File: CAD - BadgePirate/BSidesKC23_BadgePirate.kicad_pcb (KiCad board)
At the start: 2 copper layers, 54.8 x 147.9 mm, 75 parts, among them J1 UART, J2 JTAG, J3 Reset Jumper, J4 5v GND, J5 Boot Jumper, J6 USB, SW1 Boot, SW3 SW_Left, SW4 SW_Right, SW5 SW_Center, SW6 SW_Up, SW7 SW_Down, U1 CH340N, U2 ESP32-S3-WROOM-1, U3 TLV1117, U4 LTC4054, X1 sao_v169bis

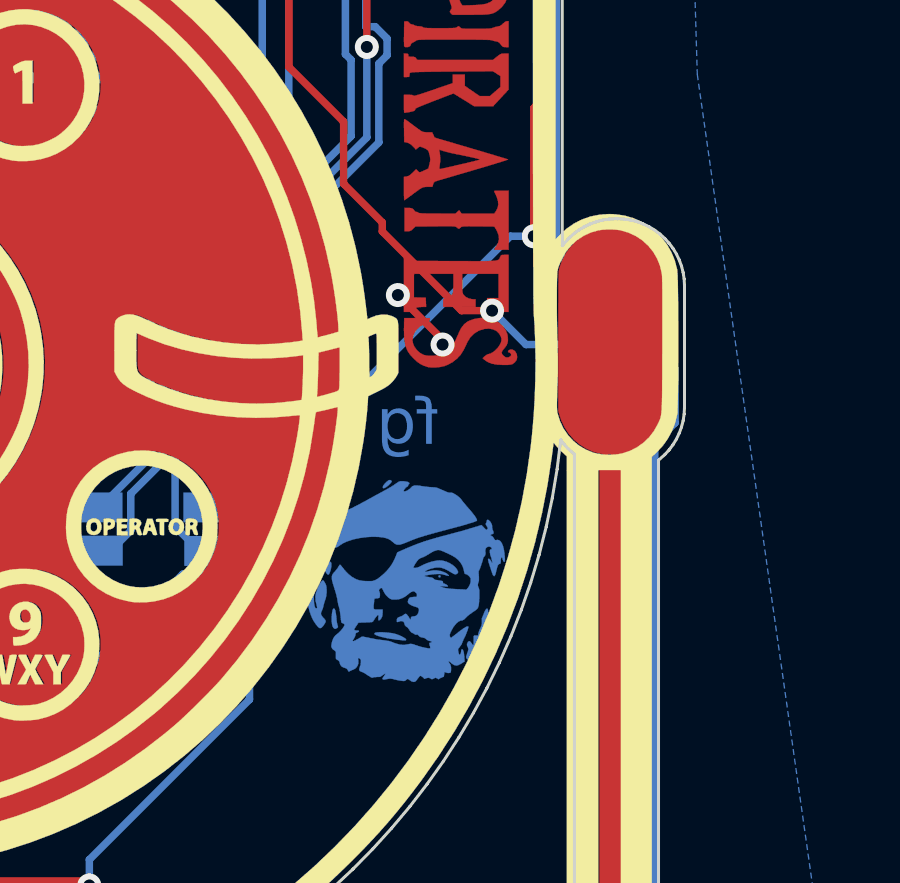
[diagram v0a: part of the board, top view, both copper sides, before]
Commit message: gerberss
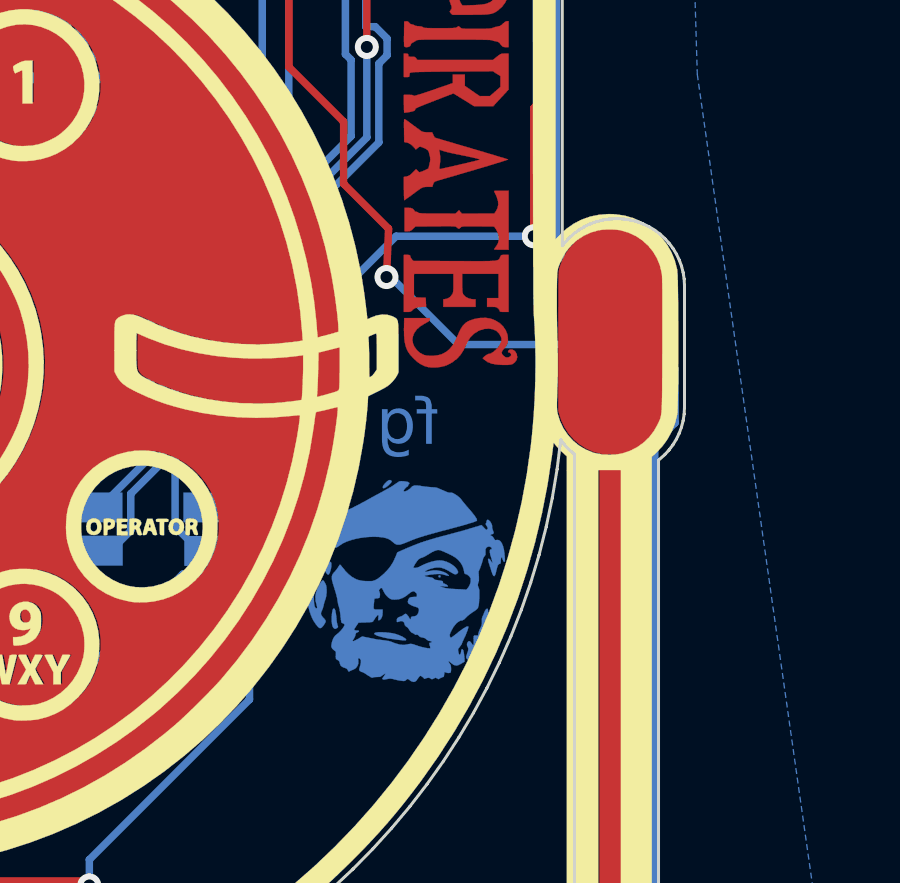
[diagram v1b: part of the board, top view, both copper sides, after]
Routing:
- net GND: track 63.5 -> 61.2 mm, vias 15 -> 13
- net IO02: track 133.7 -> 135.9 mm
- net Boot: track 152.1 -> 152.9 mm
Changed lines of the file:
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@@
   (segment (start 107.14 136.9) (end 108.1 135.94) (width 0.25) (layer "F.Cu") (net 2))
   (segment (start 112.95899 88.630416) (end 111.549074 87.2205) (width 0.25) (layer "F.Cu") (net 2))
-  (segment (start 119.43 109.5) (end 119.43 109.34) (width 0.25) (layer "F.Cu") (net 2))
   (segment (start 89.678075 172.588217) (end 89.35 172.260142) (width 0.25) (layer "F.Cu") (net 2))
   (segment (start 106.2 136.9) (end 107.14 136.9) (width 0.25) (layer "F.Cu") (net 2))
   (segment (start 81.61 79.44) (end 81.18 79.01) (width 0.25) (layer "F.Cu") (net 2))
-  (segment (start 119.43 109.34) (end 117.94 107.85) (width 0.25) (layer "F.Cu") (net 2))
   (segment (start 89.35 171.1) (end 89.82 170.63) (width 0.25) (layer "F.Cu") (net 2))
   (segment (start 100.49 49.59) (end 100.53 49.55) (width 0.25) (layer "F.Cu") (net 2))
@@
   (segment (start 89.35 172.260142) (end 89.35 171.1) (width 0.25) (layer "F.Cu") (net 2))
   (segment (start 92.268217 172.588217) (end 89.678075 172.588217) (width 0.25) (layer "F.Cu") (net 2))
-  (via (at 117.94 107.85) (size 0.8) (drill 0.4) (layers "F.Cu" "B.Cu") (free) (net 2))
   (via (at 89.82 170.63) (size 0.8) (drill 0.4) (layers "F.Cu" "B.Cu") (free) (net 2))
   (via (at 78.92 79.01) (size 0.8) (drill 0.4) (layers "F.Cu" "B.Cu") (free) (net 2))
@@
   (via (at 100.53 49.55) (size 0.8) (drill 0.4) (layers "F.Cu" "B.Cu") (free) (net 2))
   (via (at 88.63 84.41) (size 0.8) (drill 0.4) (layers "F.Cu" "B.Cu") (free) (net 2))
-  (via (at 119.43 109.5) (size 0.8) (drill 0.4) (layers "F.Cu" "B.Cu") (free) (net 2))
   (via (at 106.2 136.9) (size 0.8) (drill 0.4) (layers "F.Cu" "B.Cu") (free) (net 2))
   (via (at 111.549074 87.2205) (size 0.8) (drill 0.4) (layers "F.Cu" "B.Cu") (free) (net 2))
@@
   (segment (start 82.73 115.871517) (end 82.73 119.328041) (width 0.25) (layer "B.Cu") (net 30))
   (segment (start 82.0695 111.49) (end 81.795 111.2155) (width 0.25) (layer "B.Cu") (net 30))
+  (segment (start 102.26972 92.53) (end 102.139719 92.4) (width 0.25) (layer "F.Cu") (net 31))
+  (segment (start 117.56 107.25) (end 117.63 105.64) (width 0.25) (layer "F.Cu") (net 31))
+  (segment (start 101.3 92.4) (end 101.0255 92.6745) (width 0.25) (layer "F.Cu") (net 31))
+  (segment (start 114.31 100.25) (end 114.31 97.939595) (width 0.25) (layer "F.Cu") (net 31))
+  (segment (start 117.63 105.64) (end 116.13 104.14) (width 0.25) (layer "F.Cu") (net 31))
+  (segment (start 114.31 97.939595) (end 108.900405 92.53) (width 0.25) (layer "F.Cu") (net 31))
+  (segment (start 102.139719 92.4) (end 101.3 92.4) (width 0.25) (layer "F.Cu") (net 31))
+  (segment (start 116.13 104.14) (end 116.13 102.07) (width 0.25) (layer "F.Cu") (net 31))
+  (segment (start 116.13 102.07) (end 114.31 100.25) (width 0.25) (layer "F.Cu") (net 31))
   (segment (start 108.900405 92.53) (end 102.26972 92.53) (width 0.25) (layer "F.Cu") (net 31))
-  (segment (start 101.3 92.4) (end 101.0255 92.6745) (width 0.25) (layer "F.Cu") (net 31))
-  (segment (start 116.13 102.07) (end 114.31 100.25) (width 0.25) (layer "F.Cu") (net 31))
-  (segment (start 116.13 104.14) (end 116.13 102.07) (width 0.25) (layer "F.Cu") (net 31))
-  (segment (start 117.42 105.73) (end 117.42 105.43) (width 0.25) (layer "F.Cu") (net 31))
-  (segment (start 120.06 108.37) (end 117.42 105.73) (width 0.25) (layer "F.Cu") (net 31))
-  (segment (start 121.08 108.37) (end 120.06 108.37) (width 0.25) (layer "F.Cu") (net 31))
-  (segment (start 114.31 100.25) (end 114.31 97.939595) (width 0.25) (layer "F.Cu") (net 31))
-  (segment (start 114.31 97.939595) (end 108.900405 92.53) (width 0.25) (layer "F.Cu") (net 31))
-  (segment (start 102.26972 92.53) (end 102.139719 92.4) (width 0.25) (layer "F.Cu") (net 31))
-  (segment (start 102.139719 92.4) (end 101.3 92.4) (width 0.25) (layer "F.Cu") (net 31))
-  (segment (start 117.42 105.43) (end 116.13 104.14) (width 0.25) (layer "F.Cu") (net 31))
   (via (at 101.0255 92.6745) (size 0.8) (drill 0.4) (layers "F.Cu" "B.Cu") (net 31))
-  (via (at 121.08 108.37) (size 0.8) (drill 0.4) (layers "F.Cu" "B.Cu") (net 31))
-  (segment (start 126.503 154.1028) (end 125.355 155.2508) (width 0.25) (layer "B.Cu") (net 31))
+  (via (at 117.56 107.25) (size 0.8) (drill 0.4) (layers "F.Cu" "B.Cu") (net 31))
   (segment (start 101.0255 94.5245) (end 97.125281 98.424719) (width 0.25) (layer "B.Cu") (net 31))
   (segment (start 95.59 82.455) (end 95.59 98.705) (width 0.25) (layer "B.Cu") (net 31))
   (segment (start 96.09 59.31) (end 96.09 67.035686) (width 0.25) (layer "B.Cu") (net 31))
   (segment (start 105.08 46.705) (end 105.08 51.37) (width 0.25) (layer "B.Cu") (net 31))
+  (segment (start 127.18 112.11) (end 126.503 112.787) (width 0.25) (layer "B.Cu") (net 31))
+  (segment (start 126.503 154.1028) (end 125.355 155.2508) (width 0.25) (layer "B.Cu") (net 31))
   (segment (start 95.31 72.764) (end 95.244 72.83) (width 0.25) (layer "B.Cu") (net 31))
   (segment (start 101.045 54.355) (end 96.09 59.31) (width 0.25) (layer "B.Cu") (net 31))
-  (segment (start 127.18 110.32) (end 127.18 112.11) (width 0.25) (layer "B.Cu") (net 31))
   (segment (start 96.09 82.455) (end 95.59 82.455) (width 0.25) (layer "B.Cu") (net 31))
   (segment (start 126.36 109.5) (end 127.18 110.32) (width 0.25) (layer "B.Cu") (net 31))
-  (segment (start 126.503 112.787) (end 126.503 154.1028) (width 0.25) (layer "B.Cu") (net 31))
+  (segment (start 119.96 109.5) (end 126.36 109.5) (width 0.25) (layer "B.Cu") (net 31))
   (segment (start 104.605 45.005) (end 104.605 46.23) (width 0.25) (layer "B.Cu") (net 31))
   (segment (start 95.59 98.705) (end 95.365 98.93) (width 0.25) (layer "B.Cu") (net 31))
-  (segment (start 122.21 109.5) (end 126.36 109.5) (width 0.25) (layer "B.Cu") (net 31))
   (segment (start 105.08 51.37) (end 102.095 54.355) (width 0.25) (layer "B.Cu") (net 31))
-  (segment (start 127.18 112.11) (end 126.503 112.787) (width 0.25) (layer "B.Cu") (net 31))
   (segment (start 96.09 79.509719) (end 96.09 82.455) (width 0.25) (layer "B.Cu") (net 31))
   (segment (start 95.244 72.83) (end 94.6 72.83) (width 0.25) (layer "B.Cu") (net 31))
+  (segment (start 117.65 107.19) (end 119.96 109.5) (width 0.25) (layer "B.Cu") (net 31))
   (segment (start 94.6 78.019719) (end 96.09 79.509719) (width 0.25) (layer "B.Cu") (net 31))
   (segment (start 94.6 72.83) (end 94.6 78.019719) (width 0.25) (layer "B.Cu") (net 31))
@@
   (segment (start 102.095 54.355) (end 101.045 54.355) (width 0.25) (layer "B.Cu") (net 31))
   (segment (start 95.31 67.815686) (end 95.31 72.764) (width 0.25) (layer "B.Cu") (net 31))
+  (segment (start 127.18 110.32) (end 127.18 112.11) (width 0.25) (layer "B.Cu") (net 31))
   (segment (start 96.09 67.035686) (end 95.31 67.815686) (width 0.25) (layer "B.Cu") (net 31))
   (segment (start 95.870281 98.424719) (end 95.365 98.93) (width 0.25) (layer "B.Cu") (net 31))
-  (segment (start 121.08 108.37) (end 122.21 109.5) (width 0.25) (layer "B.Cu") (net 31))
   (segment (start 104.605 46.23) (end 105.08 46.705) (width 0.25) (layer "B.Cu") (net 31))
+  (segment (start 126.503 112.787) (end 126.503 154.1028) (width 0.25) (layer "B.Cu") (net 31))
   (segment (start 97.125281 98.424719) (end 95.870281 98.424719) (width 0.25) (layer "B.Cu") (net 31))
   (segment (start 112.34 145.02) (end 112.92 145.02) (width 0.25) (layer "F.Cu") (net 32))
@@
   (via (at 122.47 105.89) (size 0.8) (drill 0.4) (layers "F.Cu" "B.Cu") (net 60))
   (segment (start 81.395 115.491112) (end 81.395 98.93) (width 0.25) (layer "B.Cu") (net 60))
+  (segment (start 117.88 105.89) (end 112.995 110.775) (width 0.25) (layer "B.Cu") (net 60))
   (segment (start 82.0555 116.151612) (end 81.395 115.491112) (width 0.25) (layer "B.Cu") (net 60))
-  (segment (start 122.47 105.89) (end 121.69 105.89) (width 0.25) (layer "B.Cu") (net 60))
   (segment (start 107.655 126.670686) (end 107.655 127.53) (width 0.25) (layer "B.Cu") (net 60))
-  (segment (start 121.69 105.89) (end 112.995 114.585) (width 0.25) (layer "B.Cu") (net 60))
-  (segment (start 112.995 114.585) (end 112.995 121.330686) (width 0.25) (layer "B.Cu") (net 60))
   (segment (start 112.995 121.330686) (end 107.655 126.670686) (width 0.25) (layer "B.Cu") (net 60))
+  (segment (start 112.995 110.775) (end 112.995 121.330686) (width 0.25) (layer "B.Cu") (net 60))
+  (segment (start 122.47 105.89) (end 117.88 105.89) (width 0.25) (layer "B.Cu") (net 60))
   (segment (start 86.02 61.99) (end 85.97 61.99) (width 0.25) (layer "F.Cu") (net 61))
   (segment (start 92.21 38.59) (end 93.09 38.59) (width 0.25) (layer "F.Cu") (net 61))
